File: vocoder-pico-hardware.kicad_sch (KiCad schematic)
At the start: 54 parts, among them J1 Conn_02x05_Odd_Even, J2 AudioJack3_SwitchTR, J3 AudioJack3_SwitchTR, SW1 SW_Push, SW2 SW_Push, U1 TL072, U2 LM7805_TO220, U3 PCM5100A, U8 MCP6002-xMC

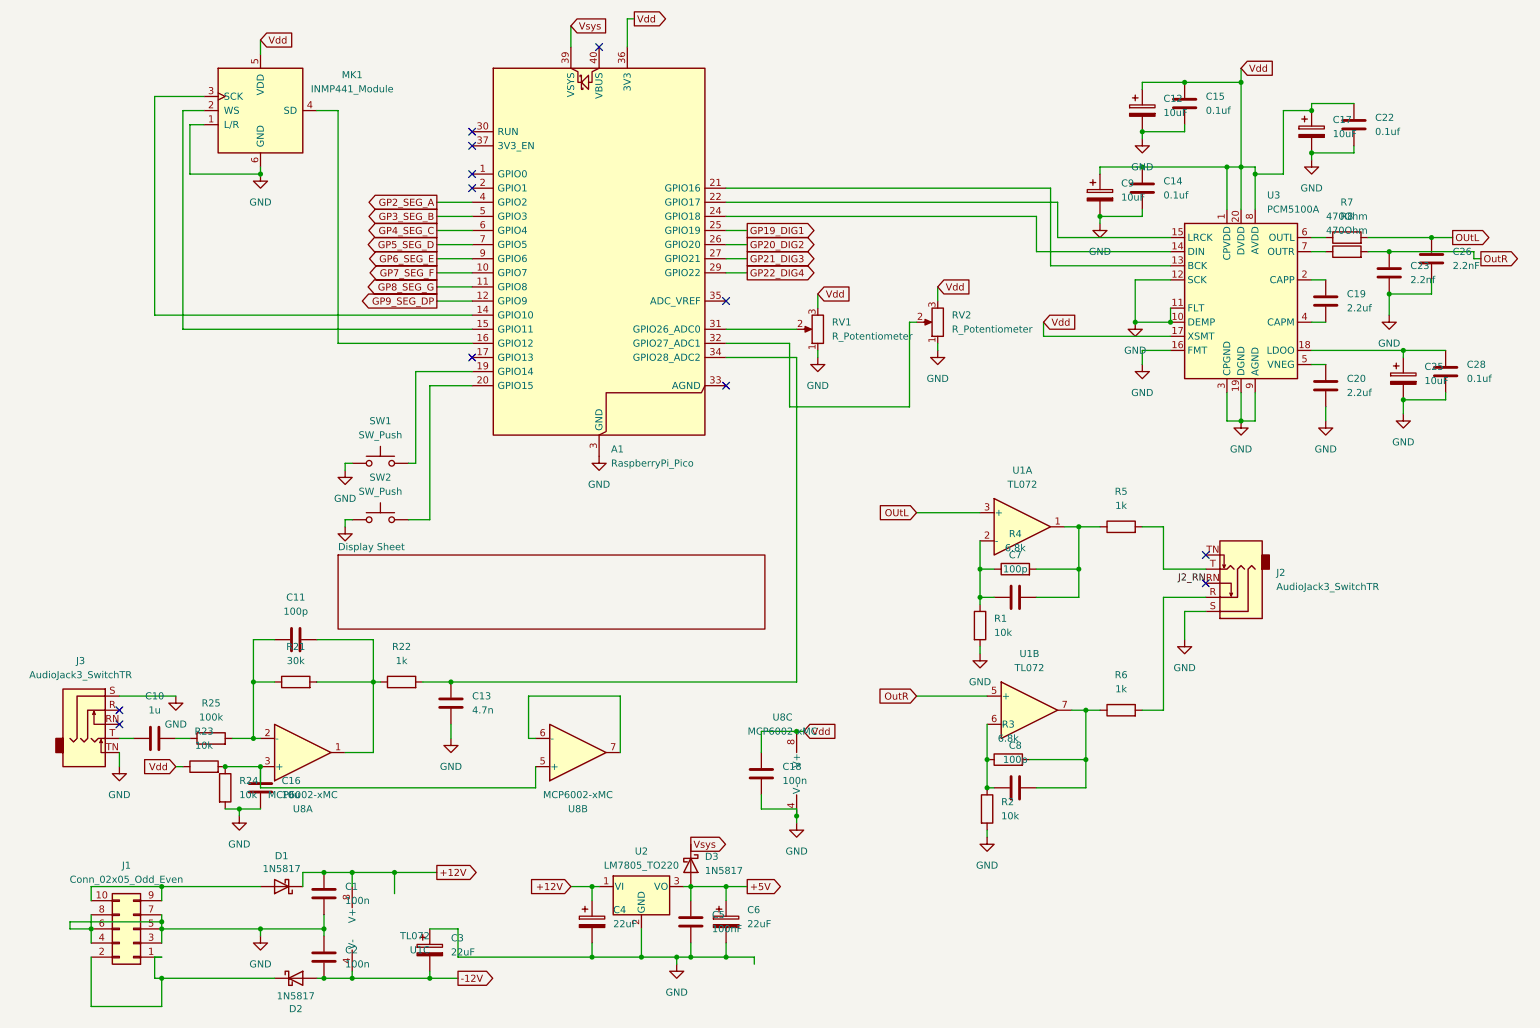
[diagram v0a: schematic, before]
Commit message: add footprints for capacitors
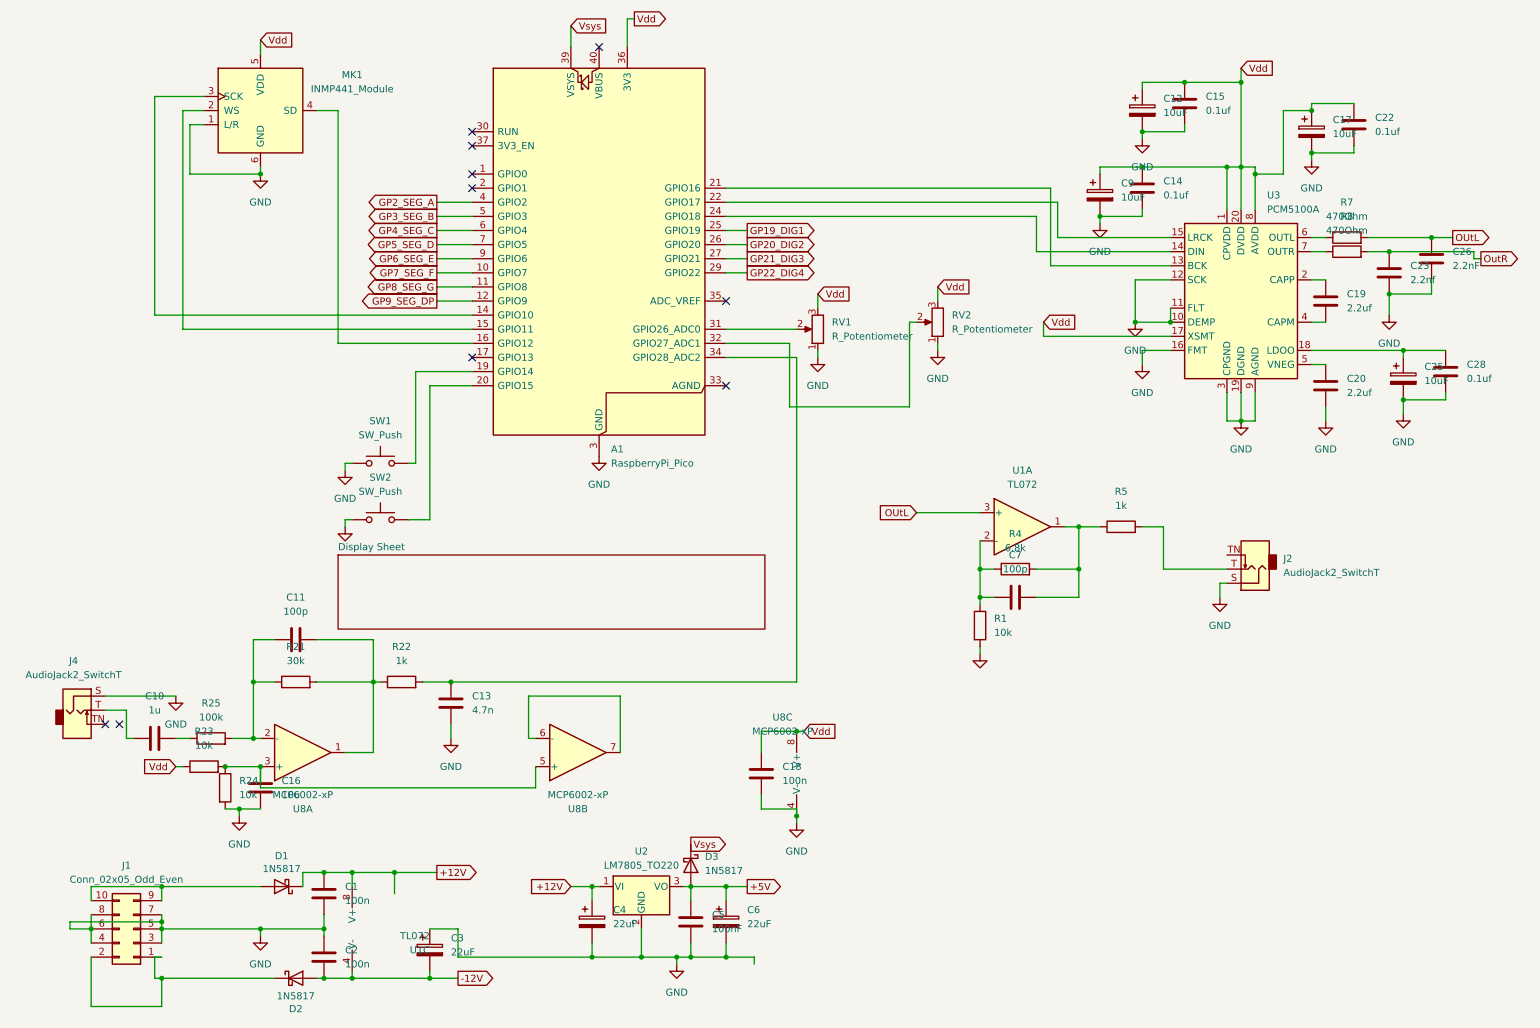
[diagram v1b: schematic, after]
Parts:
- removed C8: 100p, symbol Device:C
- removed J2, J3: AudioJack3_SwitchTR, Connector_Audio:Jack_3.5mm_QingPu_WQP-PJ398SM_Vertical_CircularHoles, symbol Connector_Audio:AudioJack3_SwitchTR
- removed R2: 10k, Resistor_THT:R_Axial_DIN0207_L6.3mm_D2.5mm_P7.62mm_Horizontal, symbol Device:R
- removed R3: 6.8k, Resistor_THT:R_Axial_DIN0207_L6.3mm_D2.5mm_P7.62mm_Horizontal, symbol Device:R
- removed R6: 1k, Resistor_THT:R_Axial_DIN0207_L6.3mm_D2.5mm_P7.62mm_Horizontal, symbol Device:R
- removed unit 2 of U1
- added J2, J4: AudioJack2_SwitchT, symbol Connector_Audio:AudioJack2_SwitchT
- U8: value MCP6002-xMC -> MCP6002-xP; footprint Package_DFN_QFN:DFN-8-1EP_3x2mm_P0.5mm_EP1.75x1.45mm -> Package_DIP:DIP-8_W7.62mm_Socket
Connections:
- net GND: now also J2.S, J4.S
- net at C10.1: now also J4.T
- net at R5.2: now also J2.T
- no-connect marks 12 -> 10
